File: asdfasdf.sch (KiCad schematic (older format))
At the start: 1 part

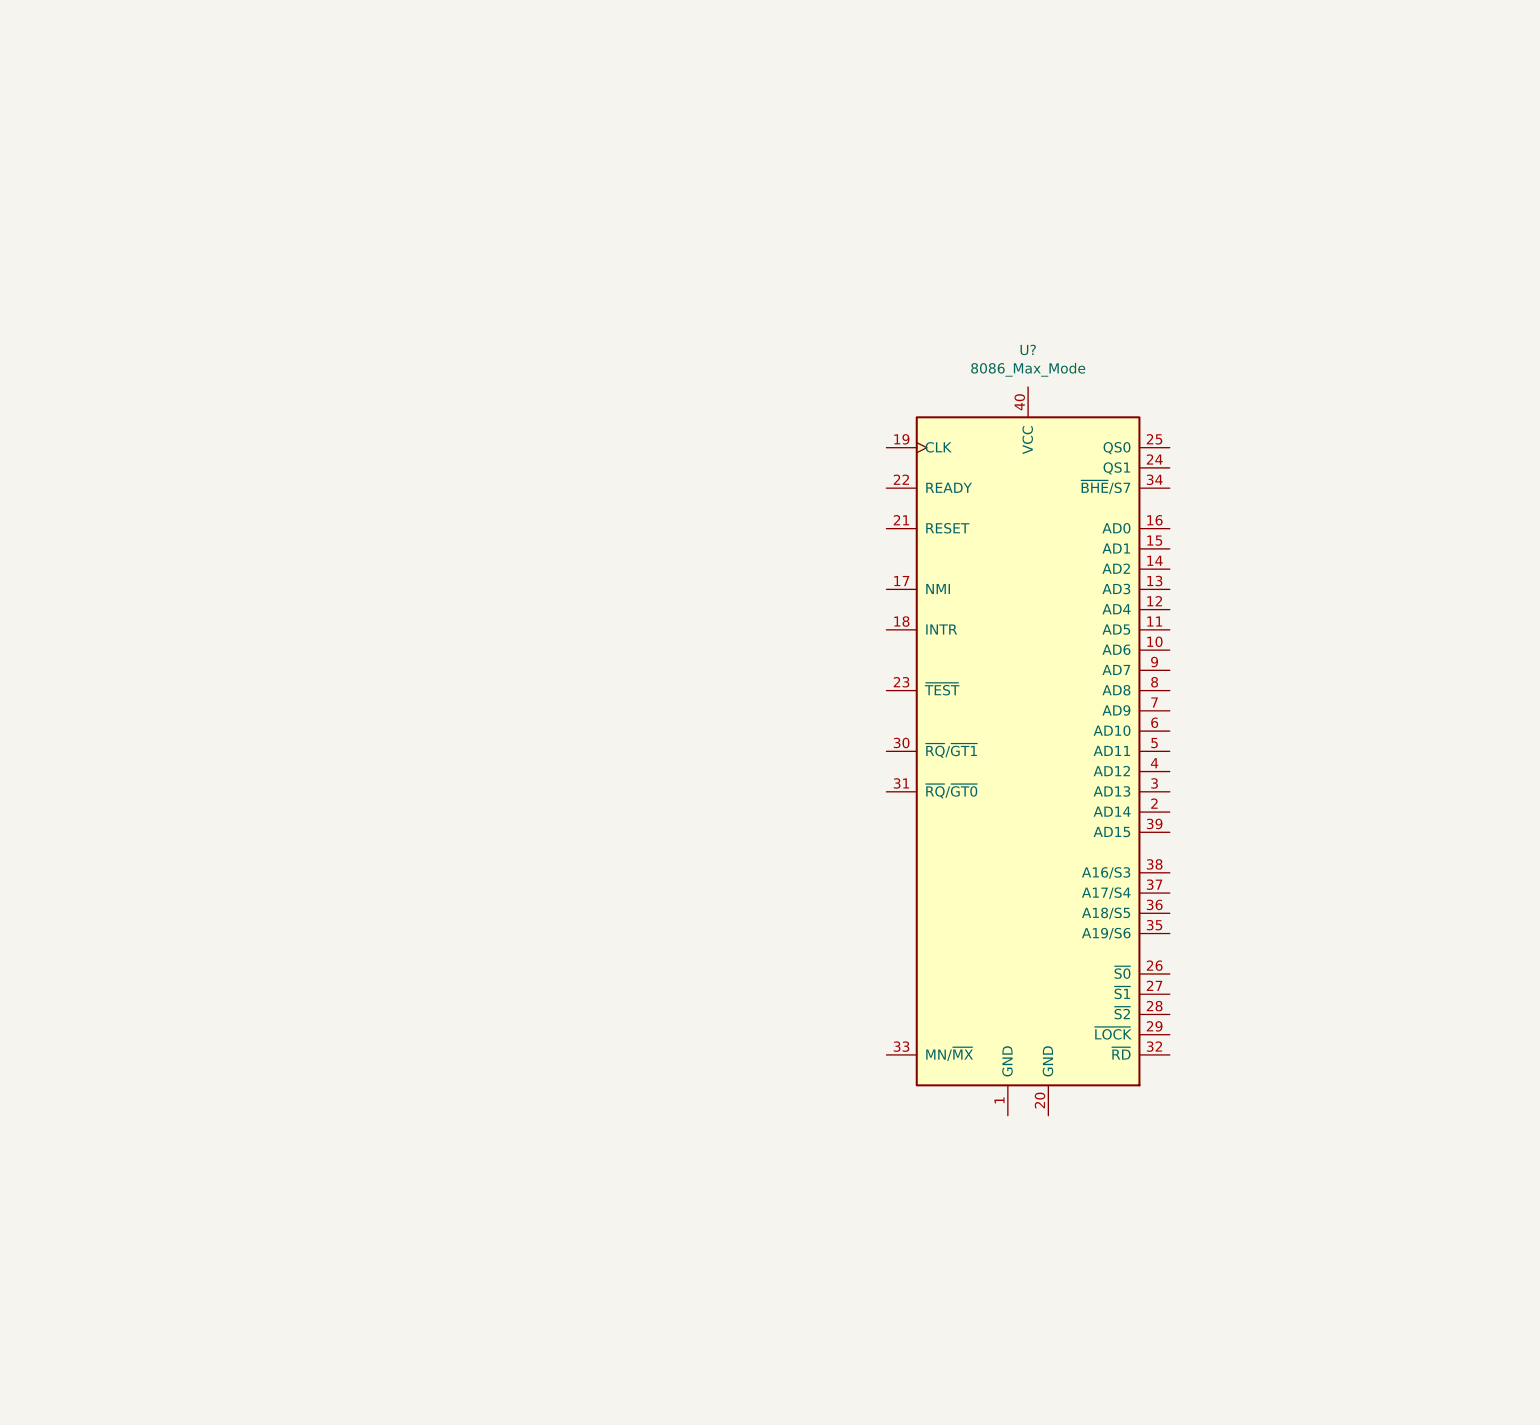
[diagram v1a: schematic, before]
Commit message: 8086 v2
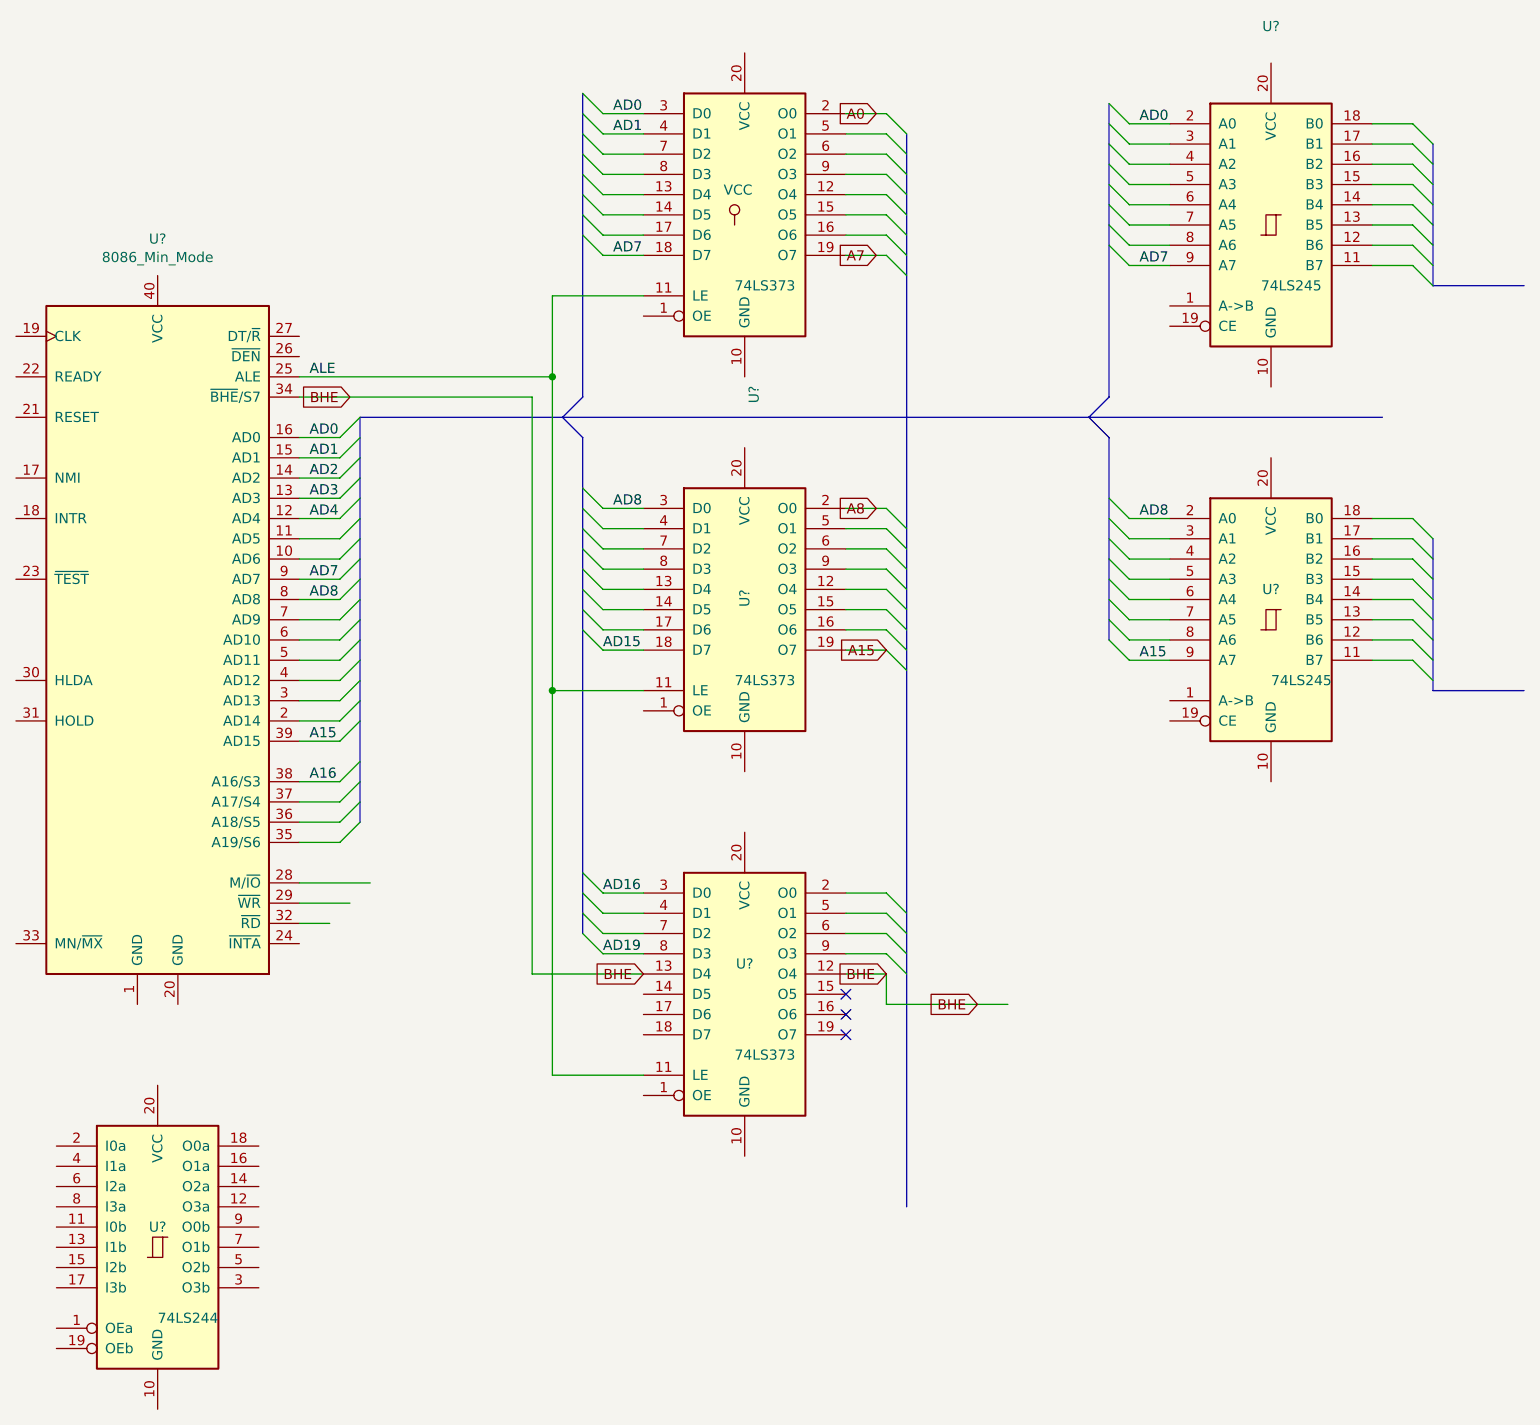
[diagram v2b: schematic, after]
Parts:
- removed U?: 8086_Max_Mode, Package_DIP:DIP-40_W15.24mm, symbol MCU_Intel:8086_Max_Mode
- added U? (x3): 74LS373, symbol 74xx:74LS373
- added U? (x2): 74LS245, symbol 74xx:74LS245
- added U?: 74LS244, symbol 74xx:74LS244
- added U?: 8086_Min_Mode, Package_DIP:DIP-40_W15.24mm, symbol MCU_Intel:8086_Min_Mode
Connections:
- new net A0: U?.2 (O0)
- new net A15: U?.19 (O7), U?.39 (AD15), U?.9 (A7)
- new net A16: U?.38 (A16/S3)
- new net A7: U?.19 (O7)
- new net A8: U?.2 (O0)
- new net AD0: U?.16 (AD0), U?.2 (A0), U?.3 (D0)
- new net AD1: U?.15 (AD1), U?.4 (D1)
- new net AD15: U?.18 (D7)
- new net AD16: U?.3 (D0)
- new net AD19: U?.8 (D3)
- new net AD2: U?.14 (AD2)
- new net AD3: U?.13 (AD3)
- new net AD4: U?.12 (AD4)
- new net AD7: U?.18 (D7), U?.9 (A7), U?.9 (AD7)
- new net AD8: U?.2 (A0), U?.3 (D0), U?.8 (AD8)
- new net ALE: U?.11 (LE), U?.11 (LE), U?.11 (LE), U?.25 (ALE)
- new net BHE: U?.12 (O4), U?.13 (D4), U?.34 (~BHE~/S7)
- no-connect marks 0 -> 3
